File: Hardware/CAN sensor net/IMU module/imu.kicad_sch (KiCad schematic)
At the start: 11 parts, among them U6 BMI088, U7 ICM-42688-P, U8 MPU-9250

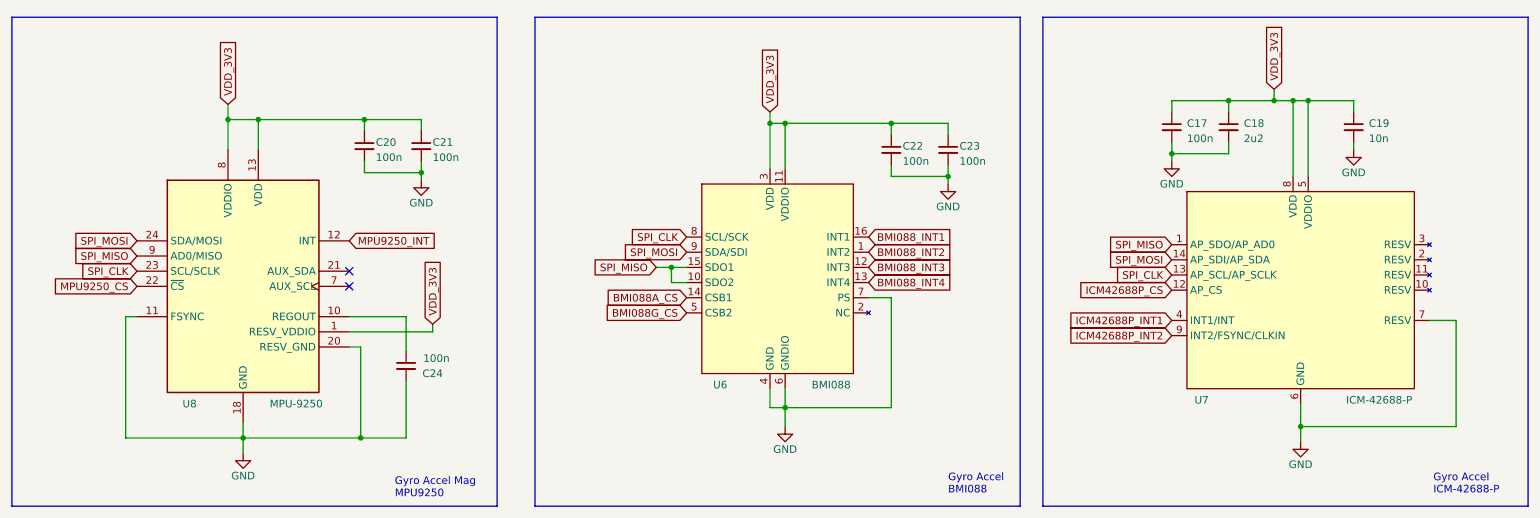
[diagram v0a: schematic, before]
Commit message: IMU production
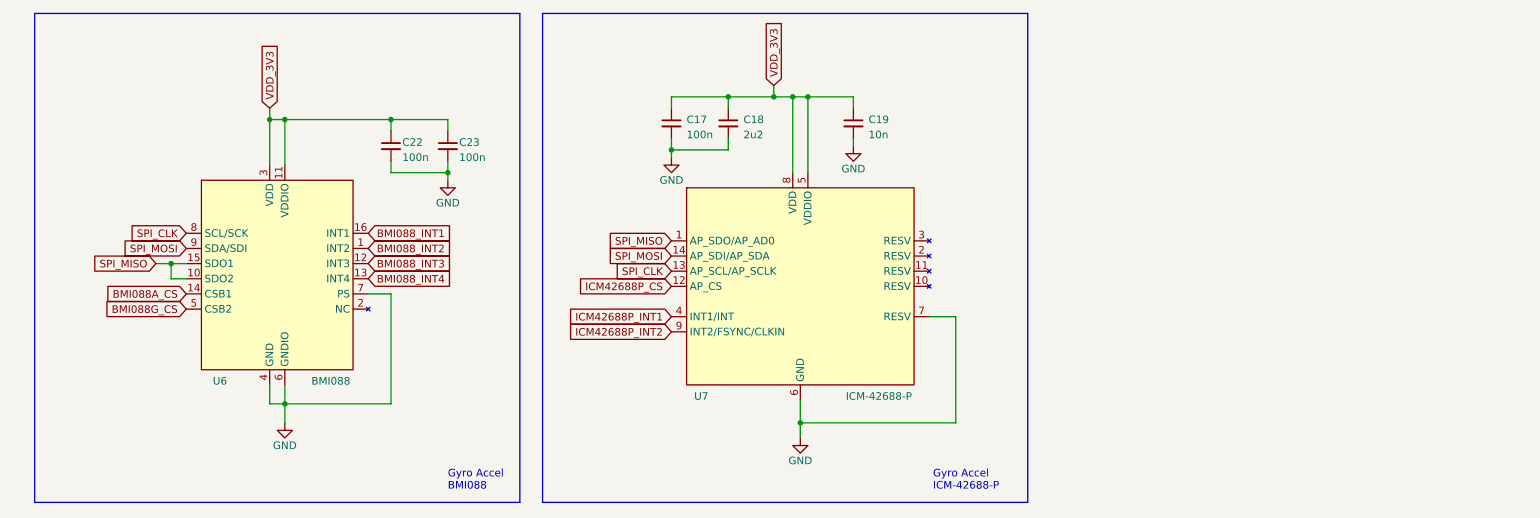
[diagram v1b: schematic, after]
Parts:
- removed C20, C21, C24: 100n, Capacitor_SMD:C_0603_1608Metric, symbol Device:C_Small
- removed U8: MPU-9250, Sensor_Motion:InvenSense_QFN-24_3x3mm_P0.4mm, symbol Sensor_Motion:MPU-9250
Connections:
- no-connect marks 2 -> 0
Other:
- note removed: "Gyro Accel Mag MPU9250"
- moved on the sheet: C17, C18, C19, C22, C23, U6, U7
